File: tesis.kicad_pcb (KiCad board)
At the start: 2 copper layers, 12 parts, among them J1 Connector_RJ10, J2 Connector_RJ10, J3 Connector_RJ10, J4 Connector_RJ10, J5 Connector_RJ10, J6 Connector_RJ10, J7 Connector_RJ10, J8 Connector_RJ10, U1 ESP32-WROOM, U2 Interface_Expansion_PCF8574, U3 Interface_Expansion_TCA9548AP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

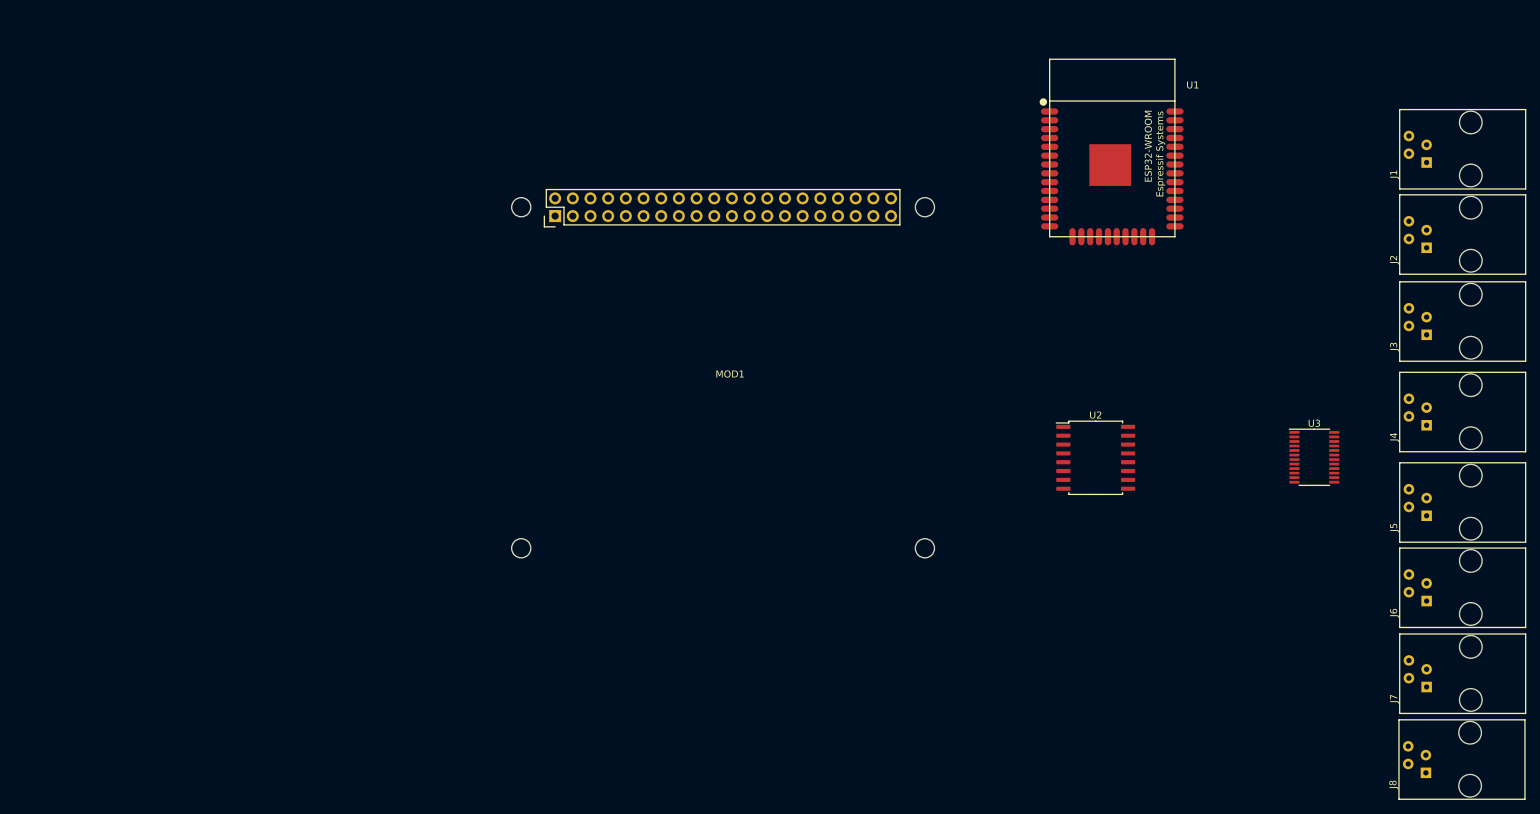
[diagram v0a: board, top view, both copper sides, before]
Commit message: Agrego v1.0 de SmartSaffron
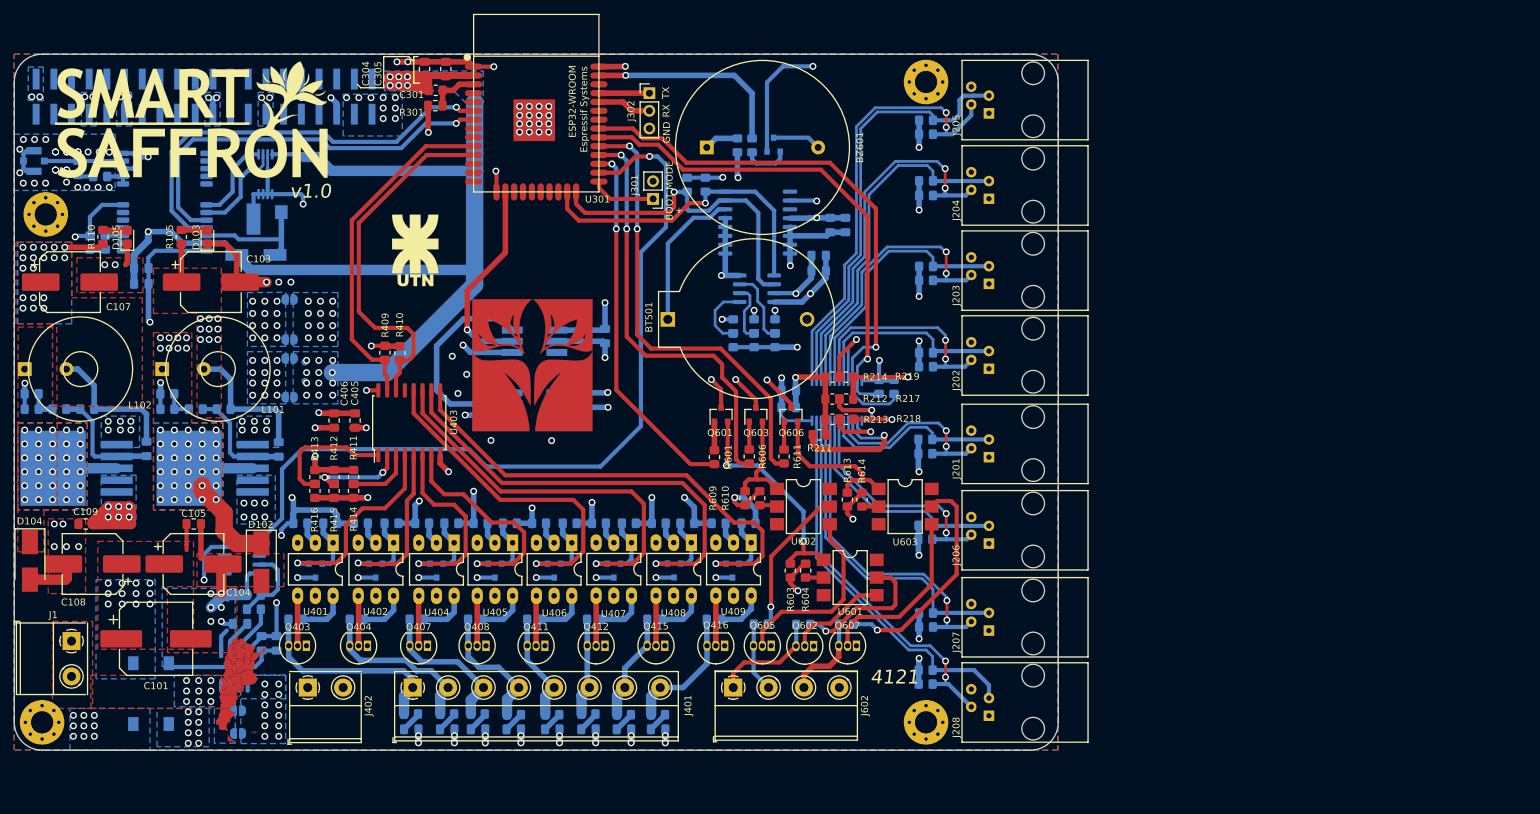
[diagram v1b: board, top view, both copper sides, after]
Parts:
- removed J2, J3, J4, J5, J6, J7, J8: Connector_RJ10, 00_lib_fp:4P4C_narrow
- removed MOD1: RPi_GPIO, 00_lib_fp:RPi_fp
- removed U3: Interface_Expansion_TCA9548APWR, Package_SO:TSSOP-24_4.4x7.8mm_P0.65mm
- added AE501: Antenna_Shield, 00_lib_fp:U.FL_Molex_MCRF_73412-0110_Vertical, B.Cu at (62.4, 58.0)
- added BT501: CR2032, 00_lib_fp:BatteryHolder_ComfortableElectronic_CH273-2450_1x2450, F.Cu at (153.5, 80.8)
- added BT502: Battery_Cell, 00_lib_fp:BatteryHolder_Seiko_MS621F, B.Cu at (96.2, 66.2)
- added BZ601: Buzzer, 00_lib_fp:Buzzer_23x10, F.Cu at (167.1, 56.1)
- added C1: 10u, 00_lib_fp:C_0805_2012Metric_Pad1.18x1.45mm_HandSolder, B.Cu at (95.2, 127.3)
- added C101: 470uF/50V, 00_lib_fp:CP_Elec_10x10, F.Cu at (80.0, 126.7)
- added C102: 33u, 00_lib_fp:C_0805_2012Metric_Pad1.18x1.45mm_HandSolder, B.Cu at (97.6, 99.5)
- added C103: 470uF/50V, 00_lib_fp:CP_Elec_8x10.5, F.Cu at (87.9, 75.4)
- added C104: 470u/50V, 00_lib_fp:CP_Elec_8x10.5, F.Cu at (85.4, 115.9)
- added C105: 1u, 00_lib_fp:C_0805_2012Metric_Pad1.18x1.45mm_HandSolder, F.Cu at (85.4, 110.2)
- added C106: 33u, 00_lib_fp:C_0805_2012Metric_Pad1.18x1.45mm_HandSolder, B.Cu at (78.6, 99.4)
- added C107: 470uF/50V, 00_lib_fp:CP_Elec_8x10.5, F.Cu at (67.6, 75.4)
- added C108: 470uF/50V, 00_lib_fp:CP_Elec_8x10.5, F.Cu at (70.9, 115.9)
- added C109: 1u, 00_lib_fp:C_0805_2012Metric_Pad1.18x1.45mm_HandSolder, F.Cu at (69.9, 110.2)
- added C2: 100n, 00_lib_fp:C_0805_2012Metric_Pad1.18x1.45mm_HandSolder, B.Cu at (97.3, 127.3)
- added C201: 10u, 00_lib_fp:C_0805_2012Metric_Pad1.18x1.45mm_HandSolder, B.Cu at (170.9, 93.4)
- added C202: 100n, 00_lib_fp:C_0805_2012Metric_Pad1.18x1.45mm_HandSolder, B.Cu at (170.9, 91.0)
- added C3: 100n, 00_lib_fp:C_0805_2012Metric_Pad1.18x1.45mm_HandSolder, B.Cu at (92.1, 124.5)
- added C301: 100n, 00_lib_fp:C_0805_2012Metric_Pad1.18x1.45mm_HandSolder, F.Cu at (120.1, 50.1)
- added C302: 100n, 00_lib_fp:C_0805_2012Metric_Pad1.18x1.45mm_HandSolder, B.Cu at (144.5, 83.2)
- added C303: 100n, 00_lib_fp:C_0805_2012Metric_Pad1.18x1.45mm_HandSolder, B.Cu at (141.1, 92.4)
- added C304: 10u, 00_lib_fp:C_0805_2012Metric_Pad1.18x1.45mm_HandSolder, F.Cu at (118.6, 44.8)
- added C305: 100n, 00_lib_fp:C_0805_2012Metric_Pad1.18x1.45mm_HandSolder, F.Cu at (121.6, 44.8)
- added C401: 100n, 00_lib_fp:C_0805_2012Metric_Pad1.18x1.45mm_HandSolder, B.Cu at (116.7, 139.7)
- added C402: 100n, 00_lib_fp:C_0805_2012Metric_Pad1.18x1.45mm_HandSolder, B.Cu at (121.8, 139.7)
- added C403: 100n, 00_lib_fp:C_0805_2012Metric_Pad1.18x1.45mm_HandSolder, B.Cu at (126.3, 139.7)
- added C404: 100n, 00_lib_fp:C_0805_2012Metric_Pad1.18x1.45mm_HandSolder, B.Cu at (131.4, 139.7)
- added C405: 10u, 00_lib_fp:C_0805_2012Metric_Pad1.18x1.45mm_HandSolder, F.Cu at (108.6, 95.3)
- added C406: 100n, 00_lib_fp:C_0805_2012Metric_Pad1.18x1.45mm_HandSolder, F.Cu at (105.6, 95.3)
- added C407: 100n, 00_lib_fp:C_0805_2012Metric_Pad1.18x1.45mm_HandSolder, B.Cu at (136.9, 139.7)
- added C408: 100n, 00_lib_fp:C_0805_2012Metric_Pad1.18x1.45mm_HandSolder, B.Cu at (142.1, 139.7)
- added C409: 100n, 00_lib_fp:C_0805_2012Metric_Pad1.18x1.45mm_HandSolder, B.Cu at (147.2, 139.7)
- added C410: 100n, 00_lib_fp:C_0805_2012Metric_Pad1.18x1.45mm_HandSolder, B.Cu at (152.1, 139.7)
- added C501: 10u, 00_lib_fp:C_0805_2012Metric_Pad1.18x1.45mm_HandSolder, B.Cu at (179.0, 67.2)
- added C502: 100n, 00_lib_fp:C_0805_2012Metric_Pad1.18x1.45mm_HandSolder, B.Cu at (176.9, 67.2)
- added C503: 10u, 00_lib_fp:C_0805_2012Metric_Pad1.18x1.45mm_HandSolder, B.Cu at (175.2, 71.6)
- added C504: 100n, 00_lib_fp:C_0805_2012Metric_Pad1.18x1.45mm_HandSolder, B.Cu at (175.2, 73.8)
- added C505: 10u, 00_lib_fp:C_0805_2012Metric_Pad1.18x1.45mm_HandSolder, B.Cu at (77.9, 75.7)
- added C506: 100n, 00_lib_fp:C_0805_2012Metric_Pad1.18x1.45mm_HandSolder, B.Cu at (77.9, 73.4)
- added D101: DF06S, 00_lib_fp:Diode_Bridge_Vishay_DFSFlat, B.Cu at (79.3, 134.6)
- added D102: 1N5824, 00_lib_fp:D_SMB_Handsoldering, F.Cu at (95.1, 115.7)
- added D103: green, 00_lib_fp:LED_0805_2012Metric_Castellated, F.Cu at (87.4, 69.0)
- added D104: 1N5824, 00_lib_fp:D_SMB_Handsoldering, F.Cu at (61.9, 115.5)
- added D105: green, 00_lib_fp:LED_0805_2012Metric_Castellated, F.Cu at (75.9, 69.0)
- added D301: WS2812, 00_lib_fp:LED_WS2812_PLCC6_5.0x5.0mm_P1.6mm, B.Cu at (134.4, 83.9)
- added D302: WS2812, 00_lib_fp:LED_WS2812_PLCC6_5.0x5.0mm_P1.6mm, B.Cu at (134.4, 92.9)
- added D501: 1N5817, 00_lib_fp:D_MiniMELF_Handsoldering, B.Cu at (94.3, 71.5)
- added D502: LED, 00_lib_fp:LED_0805_2012Metric_Castellated, B.Cu at (70.5, 69.8)
- added G1: LOGO_SSaffron, 00_lib_fp:smart_saffron, F.Cu at (85.3, 53.2)
- added G2: LOGO_utn, 00_lib_fp:logo_utn, F.Cu at (117.2, 70.5)
- added G3: LOGO_azafran, 00_lib_fp:azafran, F.Cu at (134.1, 86.6)
- added G4: LOGO_arg, 00_lib_fp:argentina, F.Cu at (92.1, 134.2)
- added J201: RJ10, 00_lib_fp:4P4C_narrow, F.Cu at (197.1, 100.6)
- added J202: RJ10, 00_lib_fp:4P4C_narrow, F.Cu at (197.1, 87.9)
- added J203: RJ10, 00_lib_fp:4P4C_narrow, F.Cu at (197.1, 75.7)
- added J204: RJ10, 00_lib_fp:4P4C_narrow, F.Cu at (197.1, 63.5)
- added J205: RJ10, 00_lib_fp:4P4C_narrow, F.Cu at (197.1, 51.2)
- added J206: RJ10, 00_lib_fp:4P4C_narrow, F.Cu at (197.1, 113.0)
- added J207: RJ10, 00_lib_fp:4P4C_narrow, F.Cu at (197.1, 125.5)
- added J208: RJ10, 00_lib_fp:4P4C_narrow, F.Cu at (197.1, 137.7)
- added J301: BOOT_Mode, 00_lib_fp:PinHeader_1x02_P2.54mm_Vertical, F.Cu at (151.4, 63.5)
- added J302: Debug_PROG, 00_lib_fp:PinHeader_1x03_P2.54mm_Vertical, F.Cu at (150.9, 48.3)
- added J401: OUTPUT_SW, 00_lib_fp:TerminalBlock_Phoenix_MKDS-1,5-8-5.08_1x08_P5.08mm_Horizontal, F.Cu at (116.9, 133.7)
- added J402: COMMON, 00_lib_fp:TerminalBlock_Phoenix_MKDS-1,5-2-5.08_1x02_P5.08mm_Horizontal, F.Cu at (101.8, 133.7)
- added J602: Lights, 00_lib_fp:TerminalBlock_Phoenix_MKDS-1,5-4-5.08_1x04_P5.08mm_Horizontal, F.Cu at (162.9, 133.7)
- added JP1: jumper, 00_lib_fp:SolderJumper-2_P1.3mm_Open_RoundedPad1.0x1.5mm, B.Cu at (91.7, 137.0)
- added JP101: jumper, 00_lib_fp:SolderJumper-2_P1.3mm_Open_RoundedPad1.0x1.5mm, B.Cu at (99.2, 83.7)
- added JP102: jumper, 00_lib_fp:SolderJumper-2_P1.3mm_Open_RoundedPad1.0x1.5mm, B.Cu at (99.2, 77.9)
- added JP103: jumper, 00_lib_fp:SolderJumper-2_P1.3mm_Open_RoundedPad1.0x1.5mm, B.Cu at (99.2, 86.4)
- added JP104: jumper, 00_lib_fp:SolderJumper-2_P1.3mm_Open_RoundedPad1.0x1.5mm, B.Cu at (99.2, 92.0)
- added JP2: jumper, 00_lib_fp:SolderJumper-2_P1.3mm_Open_RoundedPad1.0x1.5mm, B.Cu at (91.8, 140.3)
- added L101: 33uH/5A, 00_lib_fp:Coil_ferrite, F.Cu at (86.9, 87.9)
- added L102: 33uH/5A, 00_lib_fp:Coil_ferrite, F.Cu at (67.1, 87.9)
- added L501: 27u, 00_lib_fp:L_0805_2012Metric_Pad1.15x1.40mm_HandSolder, B.Cu at (68.8, 59.1)
- added MH1: MountingHole, 00_lib_fp:MountingHole_3.2mm_M3_Pad_Via, F.Cu at (63.6, 138.7)
- added MH2: MountingHole, 00_lib_fp:MountingHole_3.2mm_M3_Pad_Via, F.Cu at (190.6, 138.7)
- added MH3: MountingHole, 00_lib_fp:MountingHole_3.2mm_M3_Pad_Via, F.Cu at (64.1, 65.7)
- added MH4: MountingHole, 00_lib_fp:MountingHole_3.2mm_M3_Pad_Via, F.Cu at (190.6, 46.7)
- added MOD301: RPi_GPIO, 00_lib_fp:PinSocket_2x20_P2.54mm_Vertical_SMD, B.Cu at (86.9, 48.8)
- added Q401: bss138, 00_lib_fp:SOT-23, B.Cu at (102.9, 116.9)
- added Q402: bss138, 00_lib_fp:SOT-23, B.Cu at (111.5, 116.9)
- added Q403: mac97a8, 00_lib_fp:TO-92_Inline, F.Cu at (101.6, 127.7)
- added Q404: mac97a8, 00_lib_fp:TO-92_Inline, F.Cu at (110.4, 127.7)
- added Q405: bss138, 00_lib_fp:SOT-23, B.Cu at (120.3, 116.9)
- added Q406: bss138, 00_lib_fp:SOT-23, B.Cu at (128.7, 116.9)
- added Q407: mac97a8, 00_lib_fp:TO-92_Inline, F.Cu at (119.0, 127.7)
- added Q408: mac97a8, 00_lib_fp:TO-92_Inline, F.Cu at (127.4, 127.7)
- added Q409: bss138, 00_lib_fp:SOT-23, B.Cu at (137.2, 116.9)
- added Q410: bss138, 00_lib_fp:SOT-23, B.Cu at (145.8, 116.9)
- added Q411: mac97a8, 00_lib_fp:TO-92_Inline, F.Cu at (135.9, 127.7)
- added Q412: mac97a8, 00_lib_fp:TO-92_Inline, F.Cu at (144.5, 127.7)
- added Q413: bss138, 00_lib_fp:SOT-23, B.Cu at (154.4, 116.9)
- added Q414: bss138, 00_lib_fp:SOT-23, B.Cu at (162.8, 116.9)
- added Q415: mac97a8, 00_lib_fp:TO-92_Inline, F.Cu at (153.1, 127.7)
- added Q416: mac97a8, 00_lib_fp:TO-92_Inline, F.Cu at (161.7, 127.7)
- added Q601: bss138, 00_lib_fp:SOT-23, F.Cu at (161.2, 94.5)
- added Q602: mac97a8, 00_lib_fp:TO-92_Inline, F.Cu at (174.5, 127.7)
- added Q603: bss138, 00_lib_fp:SOT-23, F.Cu at (166.2, 94.5)
- added Q604: bss138, 00_lib_fp:SOT-23, B.Cu at (168.7, 55.7)
- added Q605: mac97a8, 00_lib_fp:TO-92_Inline, F.Cu at (168.4, 127.7)
- added Q606: bss138, 00_lib_fp:SOT-23, F.Cu at (171.2, 94.5)
- added Q607: mac97a8, 00_lib_fp:TO-92_Inline, F.Cu at (180.6, 127.7)
- added R1: R, 00_lib_fp:R_0805_2012Metric_Pad1.20x1.40mm_HandSolder, B.Cu at (94.0, 122.4)
- added R101: 1k5, 00_lib_fp:R_0805_2012Metric_Pad1.20x1.40mm_HandSolder, B.Cu at (81.6, 93.7)
- added R102: 0, 00_lib_fp:R_0805_2012Metric_Pad1.20x1.40mm_HandSolder, B.Cu at (85.7, 93.7)
- added R103: 0, 00_lib_fp:R_0805_2012Metric_Pad1.20x1.40mm_HandSolder, B.Cu at (81.6, 91.5)
- added R104: 8k2, 00_lib_fp:R_0805_2012Metric_Pad1.20x1.40mm_HandSolder, B.Cu at (89.7, 93.7)
- added R105: 2k2, 00_lib_fp:R_0805_2012Metric_Pad1.20x1.40mm_HandSolder, F.Cu at (83.6, 68.9)
- added R106: 4k7, 00_lib_fp:R_0805_2012Metric_Pad1.20x1.40mm_HandSolder, B.Cu at (62.1, 93.7)
- added R107: 0, 00_lib_fp:R_0805_2012Metric_Pad1.20x1.40mm_HandSolder, B.Cu at (66.1, 93.7)
- added R108: 0, 00_lib_fp:R_0805_2012Metric_Pad1.20x1.40mm_HandSolder, B.Cu at (62.1, 91.5)
- added R109: 15k, 00_lib_fp:R_0805_2012Metric_Pad1.20x1.40mm_HandSolder, B.Cu at (70.1, 93.7)
- added R110: 2k2, 00_lib_fp:R_0805_2012Metric_Pad1.20x1.40mm_HandSolder, F.Cu at (72.4, 68.9)
- added R2: R, 00_lib_fp:R_0805_2012Metric_Pad1.20x1.40mm_HandSolder, B.Cu at (94.0, 120.4)
- added R201: 10k, 00_lib_fp:R_0805_2012Metric_Pad1.20x1.40mm_HandSolder, B.Cu at (190.5, 100.1)
- added R202: 10k, 00_lib_fp:R_0805_2012Metric_Pad1.20x1.40mm_HandSolder, B.Cu at (190.5, 98.0)
- added R203: 10k, 00_lib_fp:R_0805_2012Metric_Pad1.20x1.40mm_HandSolder, B.Cu at (190.6, 87.6)
- added R204: 10k, 00_lib_fp:R_0805_2012Metric_Pad1.20x1.40mm_HandSolder, B.Cu at (190.6, 85.6)
- added R205: 10k, 00_lib_fp:R_0805_2012Metric_Pad1.20x1.40mm_HandSolder, B.Cu at (190.6, 75.2)
- added R206: 10k, 00_lib_fp:R_0805_2012Metric_Pad1.20x1.40mm_HandSolder, B.Cu at (190.6, 73.2)
- added R207: 4k7, 00_lib_fp:R_0805_2012Metric_Pad1.20x1.40mm_HandSolder, B.Cu at (186.0, 90.5)
- added R208: 4k7, 00_lib_fp:R_0805_2012Metric_Pad1.20x1.40mm_HandSolder, B.Cu at (183.9, 90.5)
- added R209: 10k, 00_lib_fp:R_0805_2012Metric_Pad1.20x1.40mm_HandSolder, B.Cu at (190.6, 63.0)
- added R210: 10k, 00_lib_fp:R_0805_2012Metric_Pad1.20x1.40mm_HandSolder, B.Cu at (190.6, 60.9)
- added R211: 10k, 00_lib_fp:R_0805_2012Metric_Pad1.20x1.40mm_HandSolder, F.Cu at (175.3, 97.4)
- added R212: 10k, 00_lib_fp:R_0805_2012Metric_Pad1.20x1.40mm_HandSolder, F.Cu at (177.2, 92.2)
- added R213: 10k, 00_lib_fp:R_0805_2012Metric_Pad1.20x1.40mm_HandSolder, F.Cu at (177.2, 95.1)
- added R214: 10k, 00_lib_fp:R_0805_2012Metric_Pad1.20x1.40mm_HandSolder, F.Cu at (177.2, 89.1)
- added R215: 10k, 00_lib_fp:R_0805_2012Metric_Pad1.20x1.40mm_HandSolder, B.Cu at (190.6, 54.2)
- added R216: 10k, 00_lib_fp:R_0805_2012Metric_Pad1.20x1.40mm_HandSolder, B.Cu at (190.6, 52.2)
- added R217: 10k, 00_lib_fp:R_0805_2012Metric_Pad1.20x1.40mm_HandSolder, F.Cu at (179.2, 92.2)
- added R218: 10k, 00_lib_fp:R_0805_2012Metric_Pad1.20x1.40mm_HandSolder, F.Cu at (179.2, 95.1)
- added R219: 10k, 00_lib_fp:R_0805_2012Metric_Pad1.20x1.40mm_HandSolder, F.Cu at (179.2, 89.1)
- added R220: 10k, 00_lib_fp:R_0805_2012Metric_Pad1.20x1.40mm_HandSolder, B.Cu at (190.5, 112.4)
- added R221: 10k, 00_lib_fp:R_0805_2012Metric_Pad1.20x1.40mm_HandSolder, B.Cu at (190.5, 110.4)
- added R222: 10k, 00_lib_fp:R_0805_2012Metric_Pad1.20x1.40mm_HandSolder, B.Cu at (190.6, 125.0)
- added R223: 10k, 00_lib_fp:R_0805_2012Metric_Pad1.20x1.40mm_HandSolder, B.Cu at (190.6, 123.0)
- added R224: 10k, 00_lib_fp:R_0805_2012Metric_Pad1.20x1.40mm_HandSolder, B.Cu at (190.6, 133.2)
- added R225: 10k, 00_lib_fp:R_0805_2012Metric_Pad1.20x1.40mm_HandSolder, B.Cu at (190.6, 131.2)
- added R301: 10k, 00_lib_fp:R_0805_2012Metric_Pad1.20x1.40mm_HandSolder, F.Cu at (120.2, 47.9)
- added R401: 1k, 00_lib_fp:R_0805_2012Metric_Pad1.20x1.40mm_HandSolder, B.Cu at (100.0, 123.9)
- added R402: 1k, 00_lib_fp:R_0805_2012Metric_Pad1.20x1.40mm_HandSolder, B.Cu at (108.8, 123.9)
- added R403: 470, 00_lib_fp:R_0805_2012Metric_Pad1.20x1.40mm_HandSolder, B.Cu at (116.6, 137.5)
- added R404: 470, 00_lib_fp:R_0805_2012Metric_Pad1.20x1.40mm_HandSolder, B.Cu at (121.8, 137.5)
- added R405: 1k, 00_lib_fp:R_0805_2012Metric_Pad1.20x1.40mm_HandSolder, B.Cu at (105.0, 110.1)
- added R406: 470, 00_lib_fp:R_0805_2012Metric_Pad1.20x1.40mm_HandSolder, B.Cu at (100.7, 110.1)
- added R407: 1k, 00_lib_fp:R_0805_2012Metric_Pad1.20x1.40mm_HandSolder, B.Cu at (113.8, 110.1)
- added R408: 470, 00_lib_fp:R_0805_2012Metric_Pad1.20x1.40mm_HandSolder, B.Cu at (109.4, 110.1)
- added R409: 4k7, 00_lib_fp:R_0805_2012Metric_Pad1.20x1.40mm_HandSolder, F.Cu at (112.9, 85.6)
- added R410: 4k7, 00_lib_fp:R_0805_2012Metric_Pad1.20x1.40mm_HandSolder, F.Cu at (115.0, 85.6)
- added R411: 10k, 00_lib_fp:R_0805_2012Metric_Pad1.20x1.40mm_HandSolder, F.Cu at (108.4, 103.4)
- added R412: 10k, 00_lib_fp:R_0805_2012Metric_Pad1.20x1.40mm_HandSolder, F.Cu at (105.6, 103.4)
- added R413: 10k, 00_lib_fp:R_0805_2012Metric_Pad1.20x1.40mm_HandSolder, F.Cu at (102.8, 103.4)
- added R414: 10k, 00_lib_fp:R_0805_2012Metric_Pad1.20x1.40mm_HandSolder, F.Cu at (108.4, 105.4)
- added R415: 10k, 00_lib_fp:R_0805_2012Metric_Pad1.20x1.40mm_HandSolder, F.Cu at (105.6, 105.4)
- added R416: 10k, 00_lib_fp:R_0805_2012Metric_Pad1.20x1.40mm_HandSolder, F.Cu at (102.8, 105.4)
- added R417: 1k, 00_lib_fp:R_0805_2012Metric_Pad1.20x1.40mm_HandSolder, B.Cu at (117.4, 123.9)
- added R418: 1k, 00_lib_fp:R_0805_2012Metric_Pad1.20x1.40mm_HandSolder, B.Cu at (125.8, 123.9)
- added R419: 470, 00_lib_fp:R_0805_2012Metric_Pad1.20x1.40mm_HandSolder, B.Cu at (126.2, 137.5)
- added R420: 470, 00_lib_fp:R_0805_2012Metric_Pad1.20x1.40mm_HandSolder, B.Cu at (131.4, 137.6)
- added R421: 1k, 00_lib_fp:R_0805_2012Metric_Pad1.20x1.40mm_HandSolder, B.Cu at (122.4, 110.1)
- added R422: 470, 00_lib_fp:R_0805_2012Metric_Pad1.20x1.40mm_HandSolder, B.Cu at (118.2, 110.1)
- added R423: 1k, 00_lib_fp:R_0805_2012Metric_Pad1.20x1.40mm_HandSolder, B.Cu at (130.8, 110.1)
- added R424: 470, 00_lib_fp:R_0805_2012Metric_Pad1.20x1.40mm_HandSolder, B.Cu at (126.6, 110.1)
- added R425: 1k, 00_lib_fp:R_0805_2012Metric_Pad1.20x1.40mm_HandSolder, B.Cu at (134.3, 123.9)
- added R426: 1k, 00_lib_fp:R_0805_2012Metric_Pad1.20x1.40mm_HandSolder, B.Cu at (142.9, 123.9)
- added R427: 470, 00_lib_fp:R_0805_2012Metric_Pad1.20x1.40mm_HandSolder, B.Cu at (136.9, 137.6)
- added R428: 470, 00_lib_fp:R_0805_2012Metric_Pad1.20x1.40mm_HandSolder, B.Cu at (142.1, 137.5)
- added R429: 1k, 00_lib_fp:R_0805_2012Metric_Pad1.20x1.40mm_HandSolder, B.Cu at (139.4, 110.1)
- added R430: 470, 00_lib_fp:R_0805_2012Metric_Pad1.20x1.40mm_HandSolder, B.Cu at (135.0, 110.1)
- added R431: 1k, 00_lib_fp:R_0805_2012Metric_Pad1.20x1.40mm_HandSolder, B.Cu at (147.9, 110.1)
- added R432: 470, 00_lib_fp:R_0805_2012Metric_Pad1.20x1.40mm_HandSolder, B.Cu at (143.6, 110.1)
- added R433: 1k, 00_lib_fp:R_0805_2012Metric_Pad1.20x1.40mm_HandSolder, B.Cu at (151.6, 123.9)
- added R434: 1k, 00_lib_fp:R_0805_2012Metric_Pad1.20x1.40mm_HandSolder, B.Cu at (160.1, 123.9)
- added R435: 470, 00_lib_fp:R_0805_2012Metric_Pad1.20x1.40mm_HandSolder, B.Cu at (147.2, 137.6)
- added R436: 470, 00_lib_fp:R_0805_2012Metric_Pad1.20x1.40mm_HandSolder, B.Cu at (152.1, 137.6)
- added R437: 1k, 00_lib_fp:R_0805_2012Metric_Pad1.20x1.40mm_HandSolder, B.Cu at (156.3, 110.1)
- added R438: 470, 00_lib_fp:R_0805_2012Metric_Pad1.20x1.40mm_HandSolder, B.Cu at (152.2, 110.1)
- added R439: 1k, 00_lib_fp:R_0805_2012Metric_Pad1.20x1.40mm_HandSolder, B.Cu at (165.1, 110.1)
- added R440: 470, 00_lib_fp:R_0805_2012Metric_Pad1.20x1.40mm_HandSolder, B.Cu at (160.8, 110.1)
- added R501: 1k, 00_lib_fp:R_0805_2012Metric_Pad1.20x1.40mm_HandSolder, B.Cu at (156.3, 61.4)
- added R502: 1k, 00_lib_fp:R_0805_2012Metric_Pad1.20x1.40mm_HandSolder, B.Cu at (158.9, 61.4)
- added R503: 10.5, 00_lib_fp:R_0805_2012Metric_Pad1.20x1.40mm_HandSolder, B.Cu at (72.0, 60.3)
- added R504: 1k, 00_lib_fp:R_0805_2012Metric_Pad1.20x1.40mm_HandSolder, B.Cu at (72.7, 69.8)
- added R505: 10k, 00_lib_fp:R_0805_2012Metric_Pad1.20x1.40mm_HandSolder, B.Cu at (162.9, 83.8)
- added R506: 10k, 00_lib_fp:R_0805_2012Metric_Pad1.20x1.40mm_HandSolder, B.Cu at (165.9, 83.8)
- added R507: 10k, 00_lib_fp:R_0805_2012Metric_Pad1.20x1.40mm_HandSolder, B.Cu at (168.9, 83.8)
- added R508: 10k, 00_lib_fp:R_0805_2012Metric_Pad1.20x1.40mm_HandSolder, B.Cu at (162.9, 81.8)
- added R509: 10k, 00_lib_fp:R_0805_2012Metric_Pad1.20x1.40mm_HandSolder, B.Cu at (165.9, 81.8)
- added R510: 10k, 00_lib_fp:R_0805_2012Metric_Pad1.20x1.40mm_HandSolder, B.Cu at (168.9, 81.8)
- added R601: 1k, 00_lib_fp:R_0805_2012Metric_Pad1.20x1.40mm_HandSolder, F.Cu at (160.2, 100.6)
- added R602: 1k, 00_lib_fp:R_0805_2012Metric_Pad1.20x1.40mm_HandSolder, B.Cu at (173.0, 124.6)
- added R603: 1k, 00_lib_fp:R_0805_2012Metric_Pad1.20x1.40mm_HandSolder, F.Cu at (171.1, 116.9)
- added R604: 470, 00_lib_fp:R_0805_2012Metric_Pad1.20x1.40mm_HandSolder, F.Cu at (173.3, 116.9)
- added R605: 1k, 00_lib_fp:R_0805_2012Metric_Pad1.20x1.40mm_HandSolder, B.Cu at (163.5, 55.8)
- added R606: 1k, 00_lib_fp:R_0805_2012Metric_Pad1.20x1.40mm_HandSolder, F.Cu at (165.2, 100.5)
- added R607: 1k, 00_lib_fp:R_0805_2012Metric_Pad1.20x1.40mm_HandSolder, B.Cu at (166.9, 124.6)
- added R608: 1k, 00_lib_fp:R_0805_2012Metric_Pad1.20x1.40mm_HandSolder, B.Cu at (165.6, 55.8)
- added R609: 1k, 00_lib_fp:R_0805_2012Metric_Pad1.20x1.40mm_HandSolder, F.Cu at (164.6, 106.5)
- added R610: 470, 00_lib_fp:R_0805_2012Metric_Pad1.20x1.40mm_HandSolder, F.Cu at (166.7, 106.5)
- added R611: 1k, 00_lib_fp:R_0805_2012Metric_Pad1.20x1.40mm_HandSolder, F.Cu at (170.2, 100.5)
- added R612: 1k, 00_lib_fp:R_0805_2012Metric_Pad1.20x1.40mm_HandSolder, B.Cu at (179.1, 124.6)
- added R613: 1k, 00_lib_fp:R_0805_2012Metric_Pad1.20x1.40mm_HandSolder, F.Cu at (179.3, 106.7)
- added R614: 470, 00_lib_fp:R_0805_2012Metric_Pad1.20x1.40mm_HandSolder, F.Cu at (181.4, 106.7)
- added U101: XL4005E1, 00_lib_fp:TO-263-5_TabPin3, B.Cu at (88.1, 102.2)
- added U102: XL4005E1, 00_lib_fp:TO-263-5_TabPin3, B.Cu at (68.6, 102.2)
- added U201: TCA9548APWR, 00_lib_fp:TSSOP-24_4.4x7.8mm_P0.65mm, B.Cu at (177.8, 92.5)
- added U301: ESP32-WROOM, 00_lib_fp:ESP32-WROOM, F.Cu at (134.6, 49.7)
- added U401: MOC3043, 00_lib_fp:DIP-6_W7.62mm_LongPads, F.Cu at (105.4, 112.9)
- added U402: MOC3043, 00_lib_fp:DIP-6_W7.62mm_LongPads, F.Cu at (114.1, 112.9)
- added U403: PCF8574, 00_lib_fp:SOIC-16W_7.5x10.3mm_P1.27mm, F.Cu at (116.4, 95.6)
- added U404: MOC3043, 00_lib_fp:DIP-6_W7.62mm_LongPads, F.Cu at (122.8, 112.9)
- added U405: MOC3043, 00_lib_fp:DIP-6_W7.62mm_LongPads, F.Cu at (131.2, 112.9)
- added U406: MOC3043, 00_lib_fp:DIP-6_W7.62mm_LongPads, F.Cu at (139.7, 112.9)
- added U407: MOC3043, 00_lib_fp:DIP-6_W7.62mm_LongPads, F.Cu at (148.3, 112.9)
- added U408: MOC3043, 00_lib_fp:DIP-6_W7.62mm_LongPads, F.Cu at (156.9, 112.9)
- added U409: MOC3043, 00_lib_fp:DIP-6_W7.62mm_LongPads, F.Cu at (165.5, 112.9)
- added U501: DS3231M, 00_lib_fp:SOIC-16W_7.5x10.3mm_P1.27mm, B.Cu at (166.4, 66.9)
- added U502: NEO-6M, 00_lib_fp:ublox_NEO, B.Cu at (81.2, 63.9)
- added U503: AT24C32, 00_lib_fp:TSSOP-8_4.4x3mm_P0.65mm, B.Cu at (95.7, 59.9)
- added U504: AT24C32, 00_lib_fp:SOIC-8_3.9x4.9mm_P1.27mm, B.Cu at (166.3, 76.4)
- added U601: 4N35, 00_lib_fp:SMDIP-6_W7.62mm, F.Cu at (179.7, 117.9)
- added U602: 4N35, 00_lib_fp:SMDIP-6_W7.62mm, F.Cu at (173.0, 107.7)
- added U603: 4N35, 00_lib_fp:SMDIP-6_W7.62mm, F.Cu at (187.6, 107.7)
- J1: value Connector_RJ10 -> VAC_IN; footprint 00_lib_fp:4P4C_narrow -> 00_lib_fp:TerminalBlock_Phoenix_MKDS-1,5-2-5.08_1x02_P5.08mm_Horizontal
- U1: value ESP32-WROOM -> ACS712-05; footprint 00_lib_fp:ESP32-WROOM -> 00_lib_fp:SOIC-8_3.9x4.9mm_P1.27mm; moved to B.Cu
- U2: value Interface_Expansion_PCF8574 -> LM358; footprint 00_lib_fp:SOIC-16W_7.5x10.3mm_P1.27mm -> 00_lib_fp:SOIC-8_3.9x4.9mm_P1.27mm; moved to B.Cu
- moved J1 204.1 mm to (67.8, 127.0), turned to 270 degrees
- moved U1 146.6 mm to (91.2, 131.0), turned to 90 degrees
- moved U2 123.5 mm to (92.3, 115.4), turned to 180 degrees
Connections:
- J1 pad 1: (no net) -> /monitor/[AGND_in]
- J1 pad 2: (no net) -> /[24VAC_main]
- U1 pad 1: (no net) -> /[AGND_main]
- U1 pad 2: (no net) -> /[AGND_main]
- U1 pad 3: (no net) -> /monitor/[AGND_in]
- U1 pad 4: (no net) -> /monitor/[AGND_in]
- U1 pad 5: (no net) -> GND
- U1 pad 6: (no net) -> Net-(C3-Pad1)
- U1 pad 7: (no net) -> Net-(R1-Pad1)
- U1 pad 8: (no net) -> +5V
- U2 pad 1: (no net) -> /Core/[ADC_uC]
- U2 pad 2: (no net) -> /Core/[ADC_uC]
- U2 pad 3: (no net) -> Net-(R1-Pad2)
- U2 pad 4: (no net) -> GND
- U2 pad 8: (no net) -> +5V
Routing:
- net GND: track 0.00 -> 1267.1 mm, vias 0 -> 123
- net +3V3: track 0.00 -> 679.0 mm, vias 0 -> 39
- net +5V: track 0.00 -> 385.9 mm, vias 0 -> 42
- net /[24VAC_main]: track 0.00 -> 235.3 mm, vias 0 -> 9
- net /Core/[ADC_uC]: track 0.00 -> 120.1 mm, vias 0 -> 1
- net /Core/[SDA1_uC]: track 0.00 -> 81.2 mm, vias 0 -> 1
- net /Core/[SCL1_uC]: track 0.00 -> 72.6 mm, vias 0 -> 1
- net /Outputs/P4: track 0.00 -> 68.5 mm, vias 0 -> 1
- net /Alerts/[GREEN_ALERT_in]: track 0.00 -> 65.8 mm, vias 0 -> 2
- net /inputs/SD4: track 0.00 -> 65.2 mm, vias 0 -> 2
- net /Outputs/P5: track 0.00 -> 64.3 mm, vias 0 -> 1
- net /GPS&RTC/[RX_gps]: track 0.00 -> 61.9 mm, vias 0 -> 1
- net /inputs/SC4: track 0.00 -> 61.9 mm
- net /Alerts/[YELLOW_ALERT_in]: track 0.00 -> 61.7 mm, vias 0 -> 2
- net /inputs/SD5: track 0.00 -> 58.5 mm, vias 0 -> 2
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- added copper zone on B.Cu, net (none)
- added copper zone on F.Cu, net (none)
- added copper zone on B.Cu, net +3V3
- added copper zone on PWR, net +3V3
- added copper zone on B.Cu, net +5V
- added copper zone on PWR, net +5V
- added copper zone on B.Cu, net /[24VAC_main]
- added copper zone on PWR, net /[24VAC_main]
- added copper zone on B.Cu, net /[AGND_main]
- added copper zone on PWR, net /[AGND_main]
- added copper zone on B.Cu, net /monitor/[AGND_in]
- added copper zone on F.Cu, net /monitor/[AGND_in]
- added copper zone on B.Cu, net 24V_DC
- added copper zone on F.Cu, net 24V_DC
- added copper zone on PWR, net 24V_DC
- added copper zone on B.Cu, net GND
- added copper zone on F.Cu, net GND
- added copper zone on GND, net GND
- added copper zone on B.Cu, net Net-(C102-Pad1)
- added copper zone on F.Cu, net Net-(C102-Pad1)
- added copper zone on PWR, net Net-(C102-Pad1)
- added copper zone on B.Cu, net Net-(C106-Pad1)
- added copper zone on F.Cu, net Net-(C106-Pad1)
- added copper zone on PWR, net Net-(C106-Pad1)
- added copper zone on B.Cu, net Net-(D102-Pad1)
- added copper zone on F.Cu, net Net-(D102-Pad1)
- added copper zone on B.Cu, net Net-(D104-Pad1)
- added copper zone on F.Cu, net Net-(D104-Pad1)
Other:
- board outline added: 150 x 100 mm
- copper layers 2 -> 4
- net class Default: trace_width 0.25 -> 0.4; via_dia 0.8 -> 1; via_drill 0.4 -> 0.6
- board text added: "+3V3"
- board text added: "+5V"
- board text added: "4121"
- board text added: "BOOT MODE"
- board text added: "Castro"
- board text added: "Cussa"
- board text added: "GND"
- board text added: "Grupo 6/21"
- board text added: "Navarro"
- board text added: "Nobile"
- board text added: "RX"
- board text added: "TX"
- board text added: "v1.0"
